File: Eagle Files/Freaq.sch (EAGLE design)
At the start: 30 parts, among them M1 ARDUINO-NANO-3.0

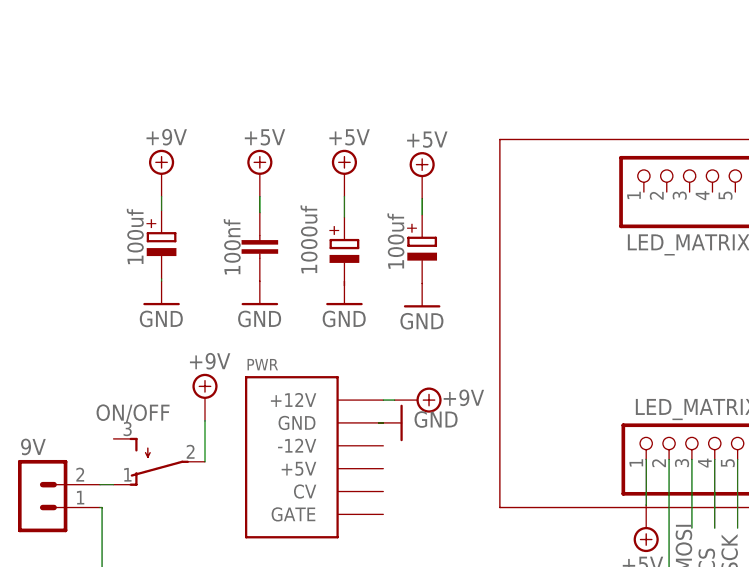
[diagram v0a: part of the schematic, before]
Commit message: updated Gerber File
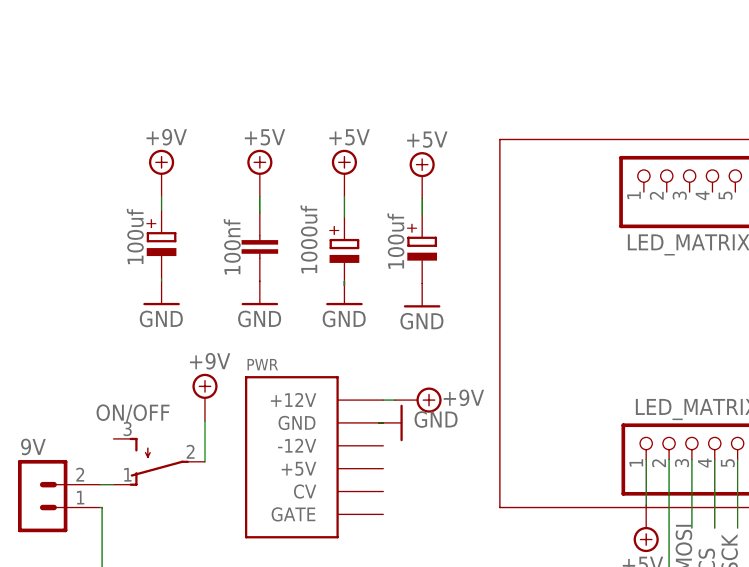
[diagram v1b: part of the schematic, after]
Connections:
- net GND: now also C5.-
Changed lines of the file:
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@@
 <wire x1="24.638" y1="55.88" x2="24.13" y2="55.88" width="0.1524" layer="91"/>
+</segment>
+<segment>
+<pinref part="C5" gate="G$1" pin="-"/>
+<pinref part="GND15" gate="1" pin="GND"/>
+<wire x1="20.32" y1="71.12" x2="20.32" y2="71.628" width="0.1524" layer="91"/>
 </segment>
 </net>
